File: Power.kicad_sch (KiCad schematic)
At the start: 15 parts, among them J1 DC JACK - (5.0x2.0 pi), U2 RT8259GJ6

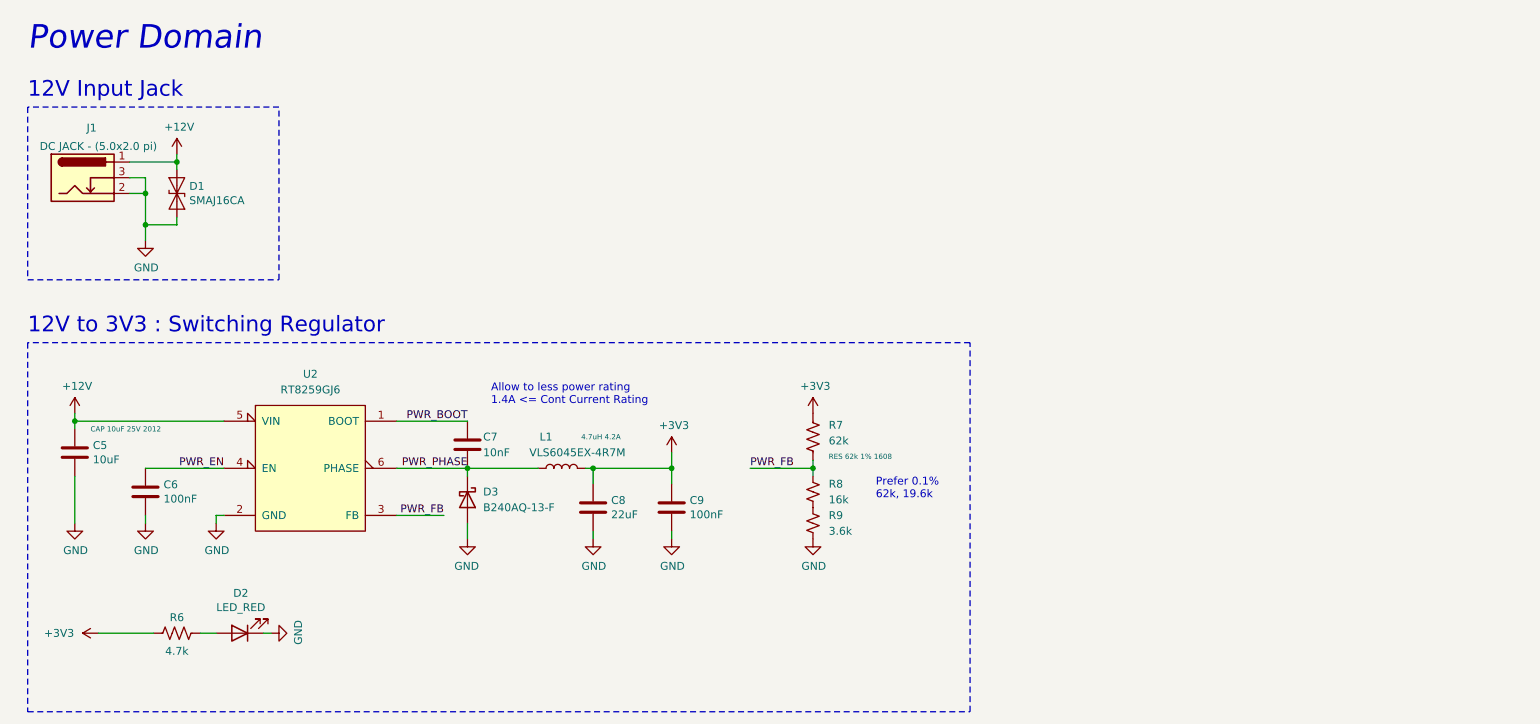
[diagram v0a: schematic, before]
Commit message: init to 0.2
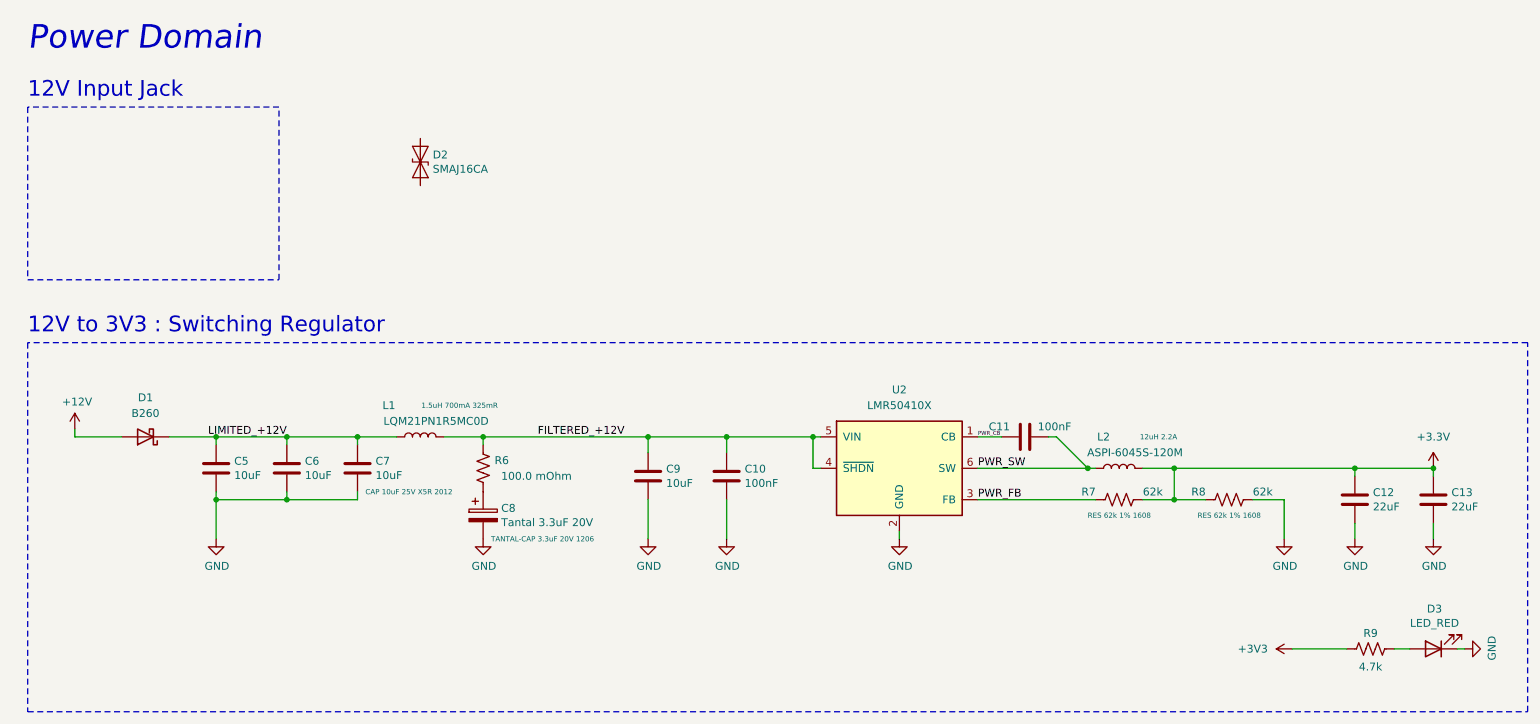
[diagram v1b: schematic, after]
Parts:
- removed C8: 22uF, Capacitor_SMD:C_0805_2012Metric, symbol Device:C
- removed D3: B240AQ-13-F, Diode_SMD:D_SMA, symbol Diode:B330
- removed J1: DC JACK - (5.0x2.0 pi), Connector_Extended_BarrelJack:BarrelJack_General_DC-012-2-5A-2.0mm, symbol Connector:Barrel_Jack_Switch
- removed R8: 16k, Resistor_SMD:R_0603_1608Metric, symbol Device:R_Small_US
- removed R9: 3.6k, Resistor_SMD:R_0603_1608Metric, symbol Device:R_Small_US
- removed U2: RT8259GJ6, Package_TO_SOT_SMD:TSOT-23-6, symbol Regulator_Switching_Extended:RT8259GJ6
- added C10, C11: 100nF, Capacitor_SMD:C_0402_1005Metric, symbol Device:C
- added C12, C13: 22uF, Capacitor_SMD:C_0805_2012Metric, symbol Device:C
- added C8: Tantal 3.3uF 20V, Capacitor_Tantalum_SMD:CP_EIA-3216-18_Kemet-A, symbol Device:C_Polarized
- added D1: B260, Diode_SMD:D_SMB, symbol Diode:B260
- added L1: LQM21PN1R5MC0D, Inductor_SMD:L_0805_2012Metric, symbol Power_Inductor_Extended:NR6028T4R7M
- added R6: 100.0 mOhm, Resistor_SMD:R_0402_1005Metric, symbol Device:R_US
- added R8: 62k, Resistor_SMD:R_0603_1608Metric, symbol Device:R_US
- added U2: LMR50410X, Package_TO_SOT_SMD:SOT-23-6, symbol Regulator_Switching:LMR14206
- C5: MFR.Part# CL21A106KAYNNNE -> GRM31CR61E106KA12L; ODR.Part# CAP 10uF 25V 2012 -> CAP 10uF 25V X5R 2012; Supplier JLCPCB-Basic -> JLCPCB-Extended
- C6, C9: value 100nF -> 10uF; footprint Capacitor_SMD:C_0402_1005Metric -> Capacitor_SMD:C_0805_2012Metric; LCSC Part C1525 -> C15850; MFR.Part# CL05B104KO5NNNC -> GRM31CR61E106KA12L; ODR.Part# CAP 100nF 1005 -> CAP 10uF 25V X5R 2012; Packaging 1005 -> 2012; Supplier JLCPCB-Basic -> JLCPCB-Extended
- C7: value 10nF -> 10uF; footprint Capacitor_SMD:C_0402_1005Metric -> Capacitor_SMD:C_0805_2012Metric; LCSC Part C15195 -> C15850; MFR.Part# CL05B103KB5NNNC -> GRM31CR61E106KA12L; ODR.Part# CAP 10nF 1005 -> CAP 10uF 25V X5R 2012; Packaging 1005 -> 2012; Supplier JLCPCB-Basic -> JLCPCB-Extended
- L2: renamed from L1; value VLS6045EX-4R7M -> ASPI-6045S-120M; LCSC Part C307880 -> C187451; MFR.Part# VLS6045EX-4R7M -> ASPI-6045S-120M; Manufacturer Taiyo Yuden -> Abracon LLC; ODR.Part# 4.7uH 4.2A -> 12uH 2.2A
- renumbered D1 to D2, D2 to D3, R6 to R9
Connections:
- net PWR_EN is gone; now on net LIMITED_+12V: C6.1
- net +12V: now also D1.2 (A); no longer C5.1, D2.1 (A1)
- net +3V3: now also R7.2, C12.1, C13.1, R8.1; no longer C9.1, R7.1
- net GND: now also C7.2, C10.2, C12.2, C13.2, C8.2, R8.2, U2.2 (GND); no longer D2.2 (A2)
- net PWR_FB: now also R7.1, U2.3 (FB); no longer R7.2
- net PWR_BOOT renamed LIMITED_+12V
- net LIMITED_+12V: now also C5.1, D1.1 (K), L1.1
- net PWR_PHASE renamed PWR_SW
- net PWR_SW: now also C11.2, U2.6 (SW); no longer C7.2
- new net: C8.1, R6.1
- new net FILTERED_+12V: C10.1, C9.1, L1.2, R6.2, U2.4 (~{SHDN}), U2.5 (VIN)
- new net PWR_CB: C11.1, U2.1 (CB)
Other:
- note removed: "Allow to less power rating 1.4A <= Cont Current Rating"
- note removed: "Prefer 0.1% 62k, 19.6k"
- moved on the sheet: C5, D2, D3, L2, R9
